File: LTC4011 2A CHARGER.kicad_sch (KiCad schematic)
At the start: 32 parts, among them J2 Conn_01x12_Pin, Q1 FQP27P06, Q2 FQP27P06, Q3 FQP27P06, Q4 IRLZ44N, U1 LTC4011CFE

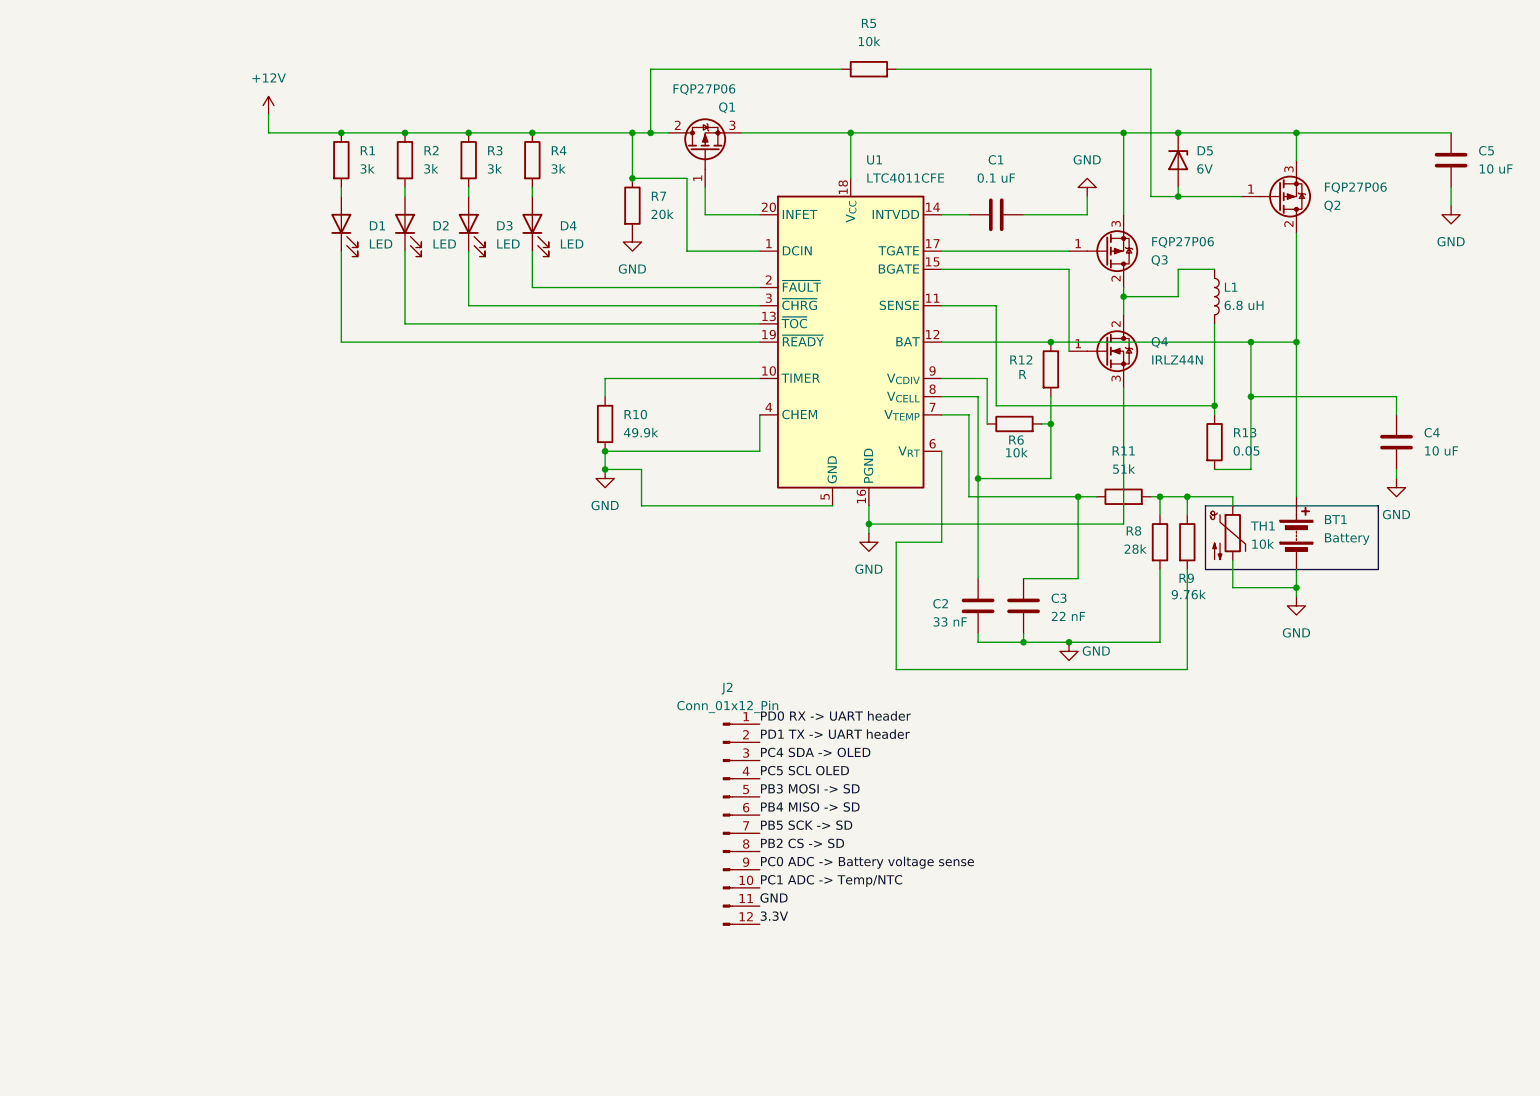
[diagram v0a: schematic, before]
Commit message: Add files via upload
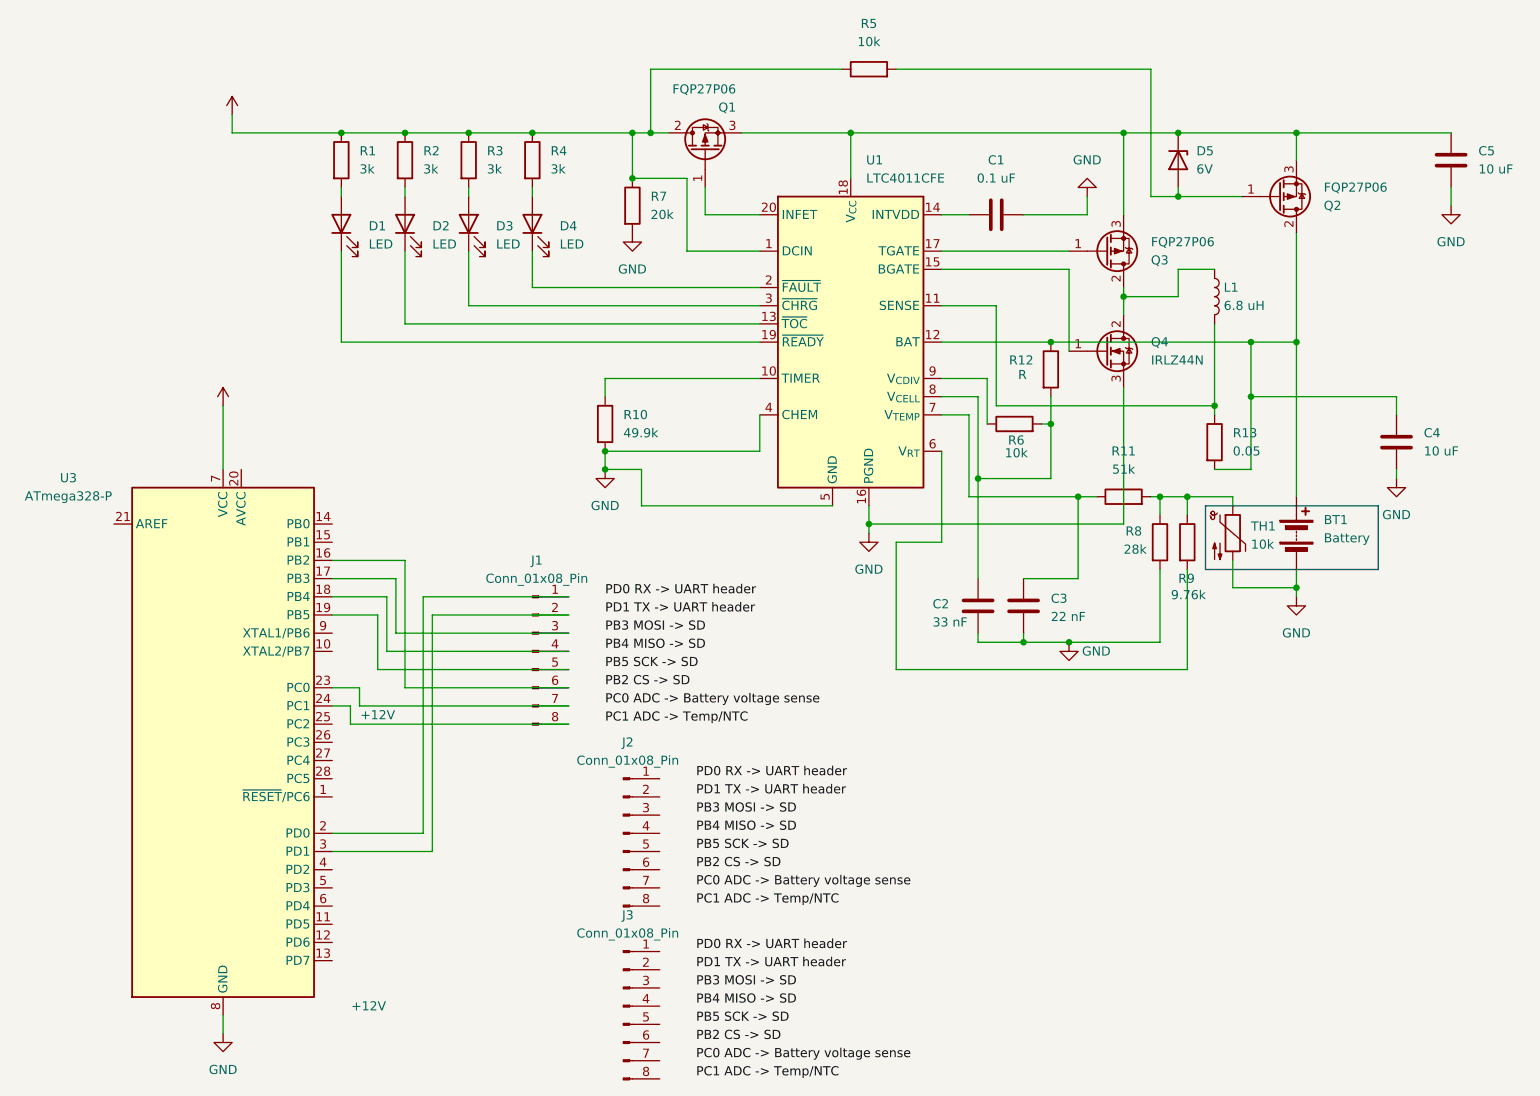
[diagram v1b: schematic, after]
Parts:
- removed J2: Conn_01x12_Pin, symbol Connector:Conn_01x12_Pin
- added J1, J2, J3: Conn_01x08_Pin, symbol Connector:Conn_01x08_Pin
- added U3: ATmega328-P, Package_DIP:DIP-28_W7.62mm, symbol MCU_Microchip_ATmega:ATmega328-P
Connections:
- net +12V: now also U3.7 (VCC)
- net GND: now also U3.22 (GND), U3.8 (GND)
- new net: J1.6 (Pin_6), U3.16 (PB2)
- new net: J1.3 (Pin_3), U3.17 (PB3)
- new net: J1.4 (Pin_4), U3.18 (PB4)
- new net: J1.5 (Pin_5), U3.19 (PB5)
- new net: J1.1 (Pin_1), U3.2 (PD0)
- new net: J1.7 (Pin_7), U3.23 (PC0)
- new net: J1.8 (Pin_8), U3.24 (PC1)
- new net: J1.2 (Pin_2), U3.3 (PD1)
